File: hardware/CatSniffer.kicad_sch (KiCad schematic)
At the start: 76 parts, among them J1 Antenna, J2 Conn_01x06_Female, J3 Conn_01x06_Female, P1 USB_C_Plug_USB2.0, SW1 SW, U1 AP2112K-3.3, U2 RFSW8006QTR7, U3 ATSAMD21E18A, U4 0900PC15A0036, U5 0900FM15D0039, U6 SW409, U7 SX1262IMLTRT, U8 CC1352P1F3RGZT, Y1 48MHz, Y2 32.768kHz, Y3 32Mhz

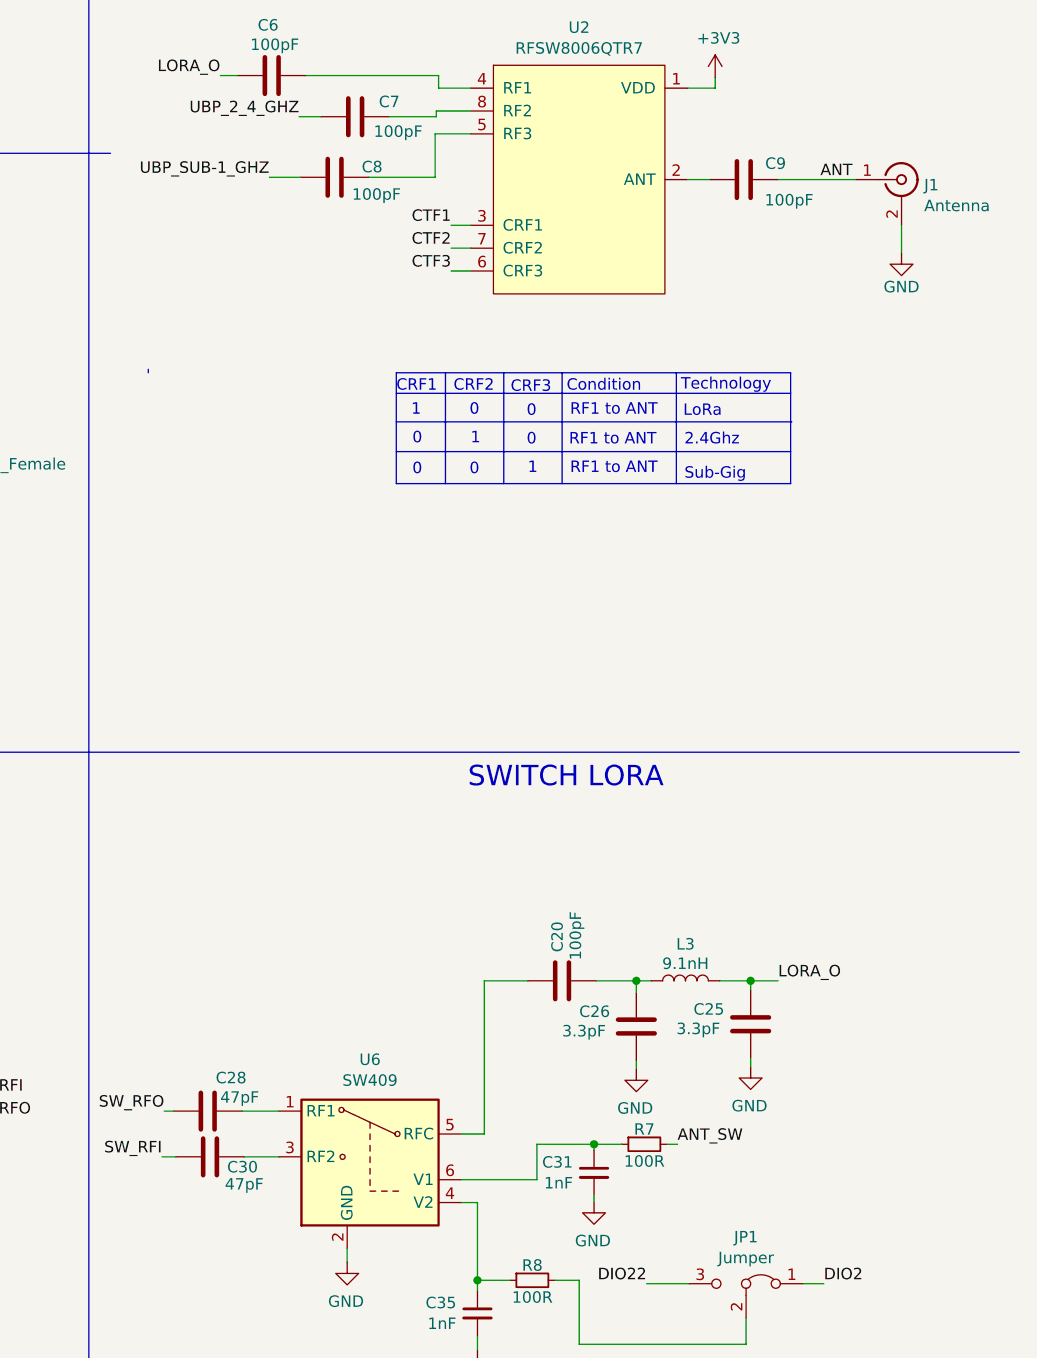
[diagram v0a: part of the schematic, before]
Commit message: update version
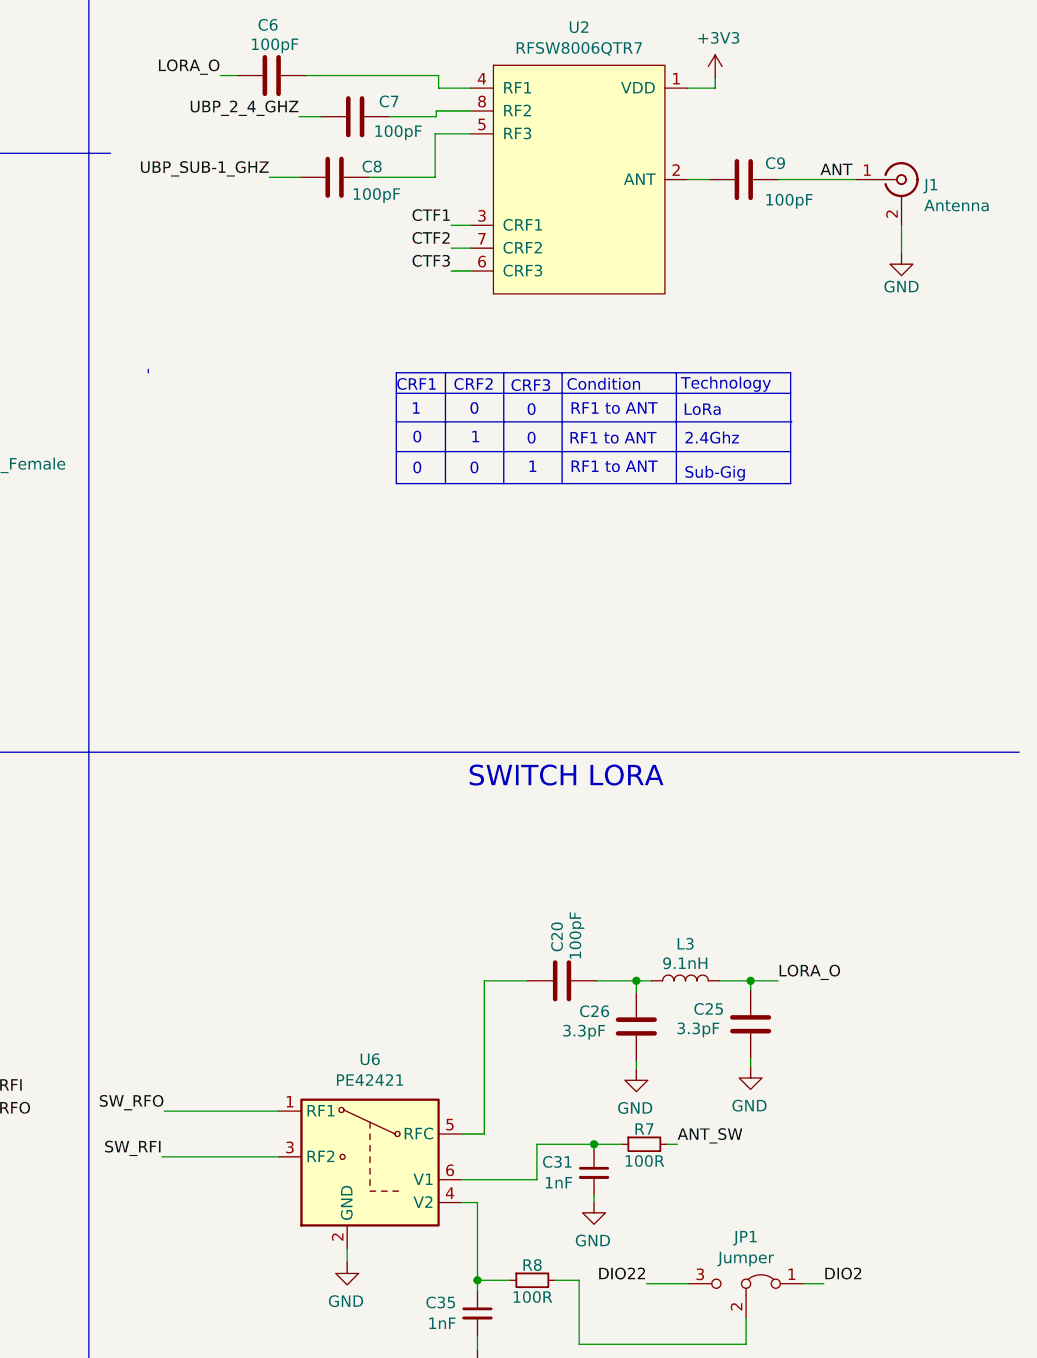
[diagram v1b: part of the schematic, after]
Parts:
- removed C28, C30: 47pF, Capacitor_SMD:C_0603_1608Metric, symbol CatSniffer-rescue:C-Device-CatStick-rescue-CatSniffer-rescue
- U6: value SW409 -> PE42421; footprint CatSniffer:SW409 -> Package_TO_SOT_SMD:SOT-363_SC-70-6; LCSC# C391968 -> -; manf# SW409 -> PE42421SCAA-Z; provedor LCSC -> Mouser
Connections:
- net SW_RFI: now also U6.3 (RF2)
- net SW_RFO: now also U6.1 (RF1)
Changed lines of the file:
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@@
     (title "CatSniffer")
     (date "2021-04-11")
-    (rev "1.0")
+    (rev "2.0")
     (company "ElectronicCats")
     (comment 3 "Edgar Herrera")
@@
     (stroke (width 0) (type default) (color 0 0 0 0))
   )
-  (wire (pts (xy 486.664 186.309) (xy 488.188 186.309))
-    (stroke (width 0) (type default) (color 0 0 0 0))
-  )
   (wire (pts (xy 303.403 50.673) (xy 316.103 50.673))
     (stroke (width 0) (type default) (color 0 0 0 0))
@@
     (stroke (width 0) (type default) (color 0 0 0 0))
   )
+  (wire (pts (xy 486.664 186.309) (xy 499.618 186.309))
+    (stroke (width 0) (type default) (color 0 0 0 0))
+  )
   (wire (pts (xy 314.198 192.024) (xy 312.039 192.024))
     (stroke (width 0) (type default) (color 0 0 0 0))
@@
     (stroke (width 0) (type default) (color 0 0 0 0))
   )
+  (wire (pts (xy 486.918 181.229) (xy 499.618 181.229))
+    (stroke (width 0) (type default) (color 0 0 0 0))
+  )
   (wire (pts (xy 548.64 166.751) (xy 552.069 166.751))
     (stroke (width 0) (type default) (color 0 0 0 0))
@@
     (stroke (width 0) (type default) (color 0 0 0 0))
   )
-  (wire (pts (xy 495.554 181.229) (xy 499.618 181.229))
-    (stroke (width 0) (type default) (color 0 0 0 0))
-  )
   (wire (pts (xy 357.124 169.164) (xy 357.124 164.719))
     (stroke (width 0) (type default) (color 0 0 0 0))
   )
-  (wire (pts (xy 495.808 186.309) (xy 499.618 186.309))
-    (stroke (width 0) (type default) (color 0 0 0 0))
-  )
   (polyline (pts (xy 531.114 99.187) (xy 531.114 111.506))
     (stroke (width 0) (type default) (color 0 0 0 0))
@@
     (stroke (width 0) (type default) (color 0 0 0 0))
   )
-  (wire (pts (xy 486.918 181.229) (xy 487.934 181.229))
-    (stroke (width 0) (type default) (color 0 0 0 0))
-  )
   (wire (pts (xy 177.038 166.37) (xy 172.339 166.37))
     (stroke (width 0) (type default) (color 0 0 0 0))
@@
     (pin "1")
   )
-  (symbol (lib_id "CatSniffer-rescue:C-Device-CatStick-rescue-CatSniffer-rescue") (at 491.744 181.229 90) (unit 1)
-    (in_bom yes) (on_board yes)
-    (property "Reference" "C28" (id 0) (at 496.062 177.546 90)
-      (effects (font (size 1.27 1.27)) (justify left))
-    )
-    (property "Value" "47pF" (id 1) (at 497.459 179.705 90)
-      (effects (font (size 1.27 1.27)) (justify left))
-    )
-    (property "Footprint" "Capacitor_SMD:C_0603_1608Metric" (id 2) (at 495.554 180.2638 0)
-      (effects (font (size 1.27 1.27)) hide)
-    )
-    (property "Datasheet" "" (id 3) (at 491.744 181.229 0))
-    (property "provedor" "LCSC" (id 4) (at 491.744 181.229 0)
-      (effects (font (size 1.27 1.27)) hide)
-    )
-    (property "LCSC#" "C519486" (id 5) (at 491.744 181.229 0)
-      (effects (font (size 1.27 1.27)) hide)
-    )
-    (property "manf#" "CC0603FRNPO9BN470" (id 6) (at 491.744 181.229 0)
-      (effects (font (size 1.27 1.27)) hide)
-    )
-    (pin "1")
-    (pin "2")
-  )
-  (symbol (lib_id "CatSniffer-rescue:C-Device-CatStick-rescue-CatSniffer-rescue") (at 491.998 186.309 90) (unit 1)
-    (in_bom yes) (on_board yes)
-    (property "Reference" "C30" (id 0) (at 497.332 187.452 90)
-      (effects (font (size 1.27 1.27)) (justify left))
-    )
-    (property "Value" "47pF" (id 1) (at 497.967 189.357 90)
-      (effects (font (size 1.27 1.27)) (justify left))
-    )
-    (property "Footprint" "Capacitor_SMD:C_0603_1608Metric" (id 2) (at 495.808 185.3438 0)
-      (effects (font (size 1.27 1.27)) hide)
-    )
-    (property "Datasheet" "" (id 3) (at 491.998 186.309 0))
-    (property "provedor" "LCSC" (id 4) (at 491.998 186.309 0)
-      (effects (font (size 1.27 1.27)) hide)
-    )
-    (property "LCSC#" "C519486" (id 5) (at 491.998 186.309 0)
-      (effects (font (size 1.27 1.27)) hide)
-    )
-    (property "manf#" "CC0603FRNPO9BN470" (id 6) (at 491.998 186.309 0)
-      (effects (font (size 1.27 1.27)) hide)
-    )
-    (pin "1")
-    (pin "2")
-  )
   (symbol (lib_id "CatSniffer-rescue:C-Device-CatStick-rescue-CatSniffer-rescue") (at 539.369 171.831 0) (unit 1)
     (in_bom yes) (on_board yes)
@@
     (in_bom yes) (on_board yes)
     (property "Reference" "U6" (id 0) (at 509.778 175.514 0))
-    (property "Value" "SW409" (id 1) (at 509.778 177.8254 0))
-    (property "Footprint" "CatSniffer:SW409" (id 2) (at 509.778 183.769 0)
+    (property "Value" "PE42421" (id 1) (at 509.778 177.8254 0))
+    (property "Footprint" "Package_TO_SOT_SMD:SOT-363_SC-70-6" (id 2) (at 509.778 183.769 0)
       (effects (font (size 1.27 1.27)) hide)
     )
-    (property "Datasheet" "https://datasheet.lcsc.com/lcsc/1912111437_RFIC-SW409_C391968.pdf" (id 3) (at 509.778 183.769 0)
+    (property "Datasheet" "https://www.mouser.mx/datasheet/2/281/pe42421ds-1671115.pdf" (id 3) (at 509.778 183.769 0)
       (effects (font (size 1.27 1.27)) hide)
     )
-    (property "LCSC#" "C391968" (id 4) (at 509.778 186.309 0)
+    (property "LCSC#" "-" (id 4) (at 509.778 186.309 0)
       (effects (font (size 1.27 1.27)) hide)
     )
-    (property "manf#" "SW409" (id 5) (at 509.778 186.309 0)
+    (property "manf#" "PE42421SCAA-Z" (id 5) (at 509.778 186.309 0)
       (effects (font (size 1.27 1.27)) hide)
     )
-    (property "provedor" "LCSC" (id 6) (at 509.778 186.309 0)
+    (property "provedor" "Mouser" (id 6) (at 509.778 186.309 0)
       (effects (font (size 1.27 1.27)) hide)
     )
@@
       (reference "C27") (unit 1) (value "100pF") (footprint "Capacitor_SMD:C_0603_1608Metric")
     )
-    (path "/00000000-0000-0000-0000-000060977a2f"
-      (reference "C28") (unit 1) (value "47pF") (footprint "Capacitor_SMD:C_0603_1608Metric")
-    )
     (path "/00000000-0000-0000-0000-000060ea4035"
       (reference "C29") (unit 1) (value "0.1uF") (footprint "Capacitor_SMD:C_0603_1608Metric")
     )
-    (path "/00000000-0000-0000-0000-000060977e80"
-      (reference "C30") (unit 1) (value "47pF") (footprint "Capacitor_SMD:C_0603_1608Metric")
-    )
     (path "/00000000-0000-0000-0000-000060cf4963"
       (reference "C31") (unit 1) (value "1nF") (footprint "Capacitor_SMD:C_0603_1608Metric")
@@
     )
     (path "/00000000-0000-0000-0000-000060fa8e32"
-      (reference "U6") (unit 1) (value "SW409") (footprint "CatSniffer:SW409")
+      (reference "U6") (unit 1) (value "PE42421") (footprint "Package_TO_SOT_SMD:SOT-363_SC-70-6")
     )
     (path "/00000000-0000-0000-0000-000060bf3807"

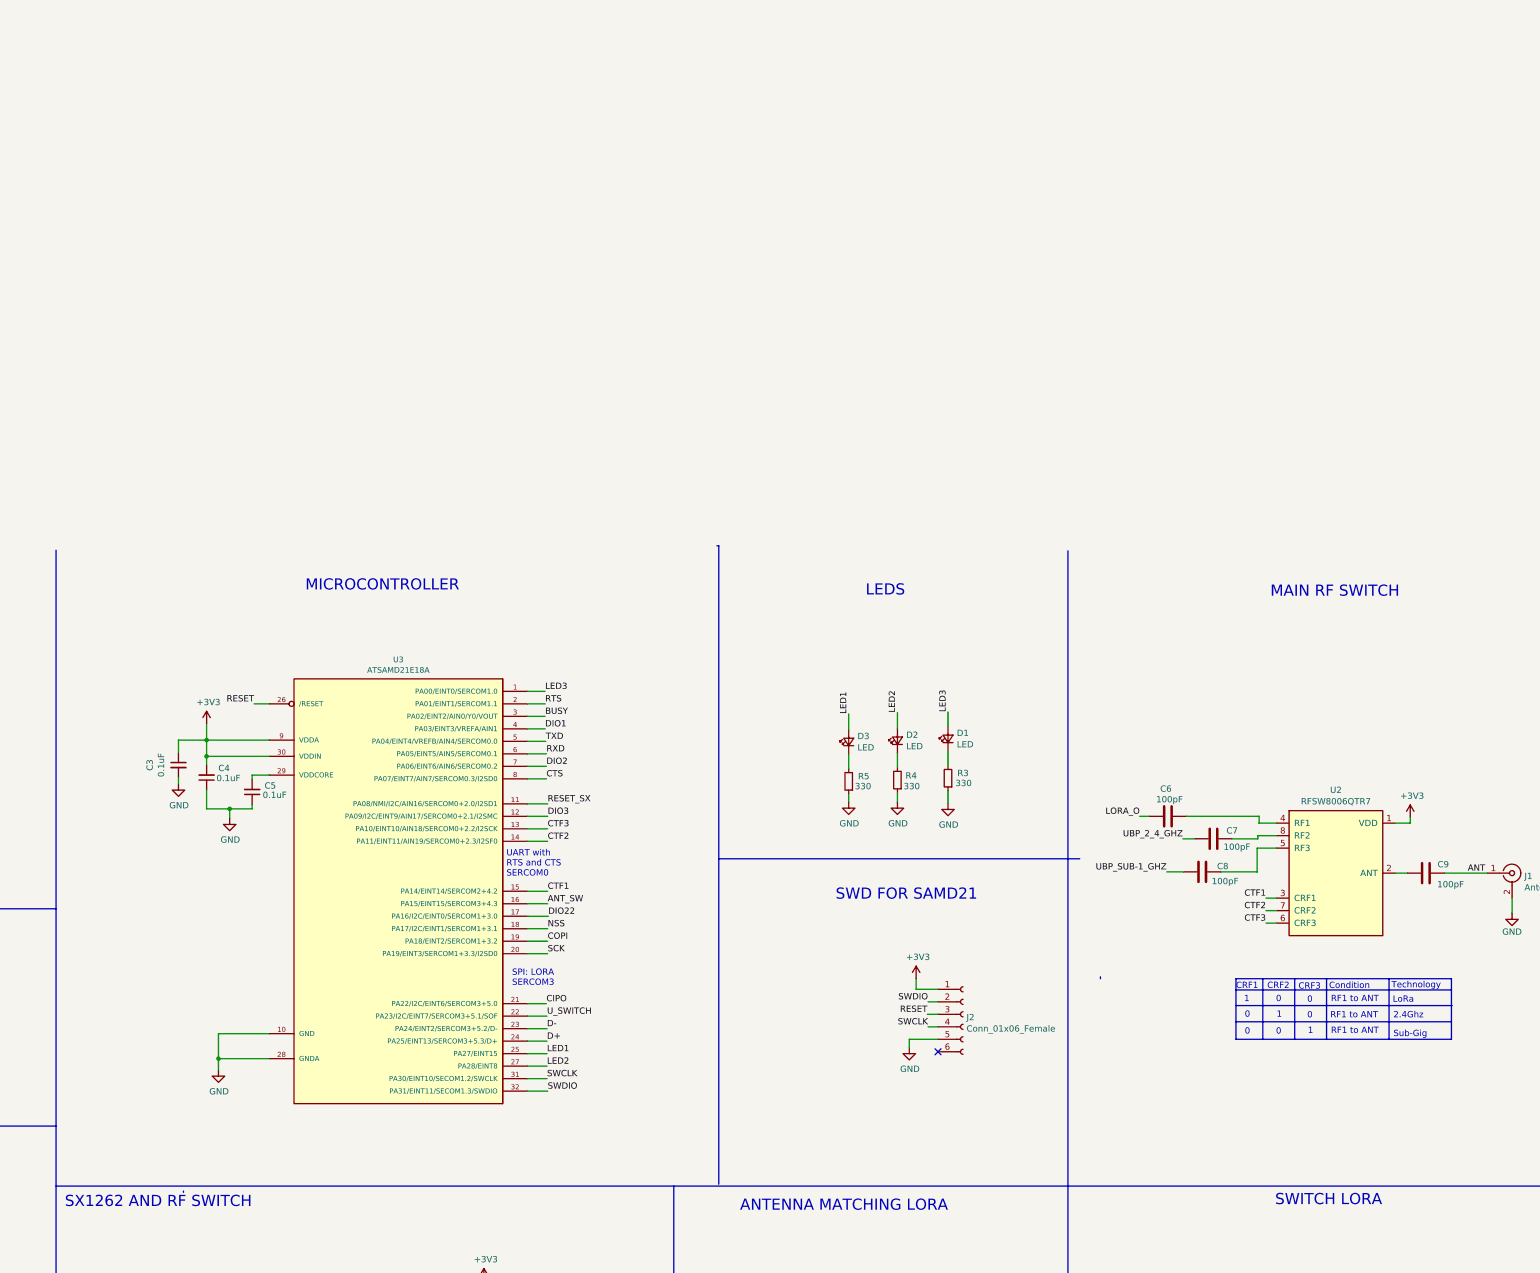
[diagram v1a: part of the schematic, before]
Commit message: Init RP2040
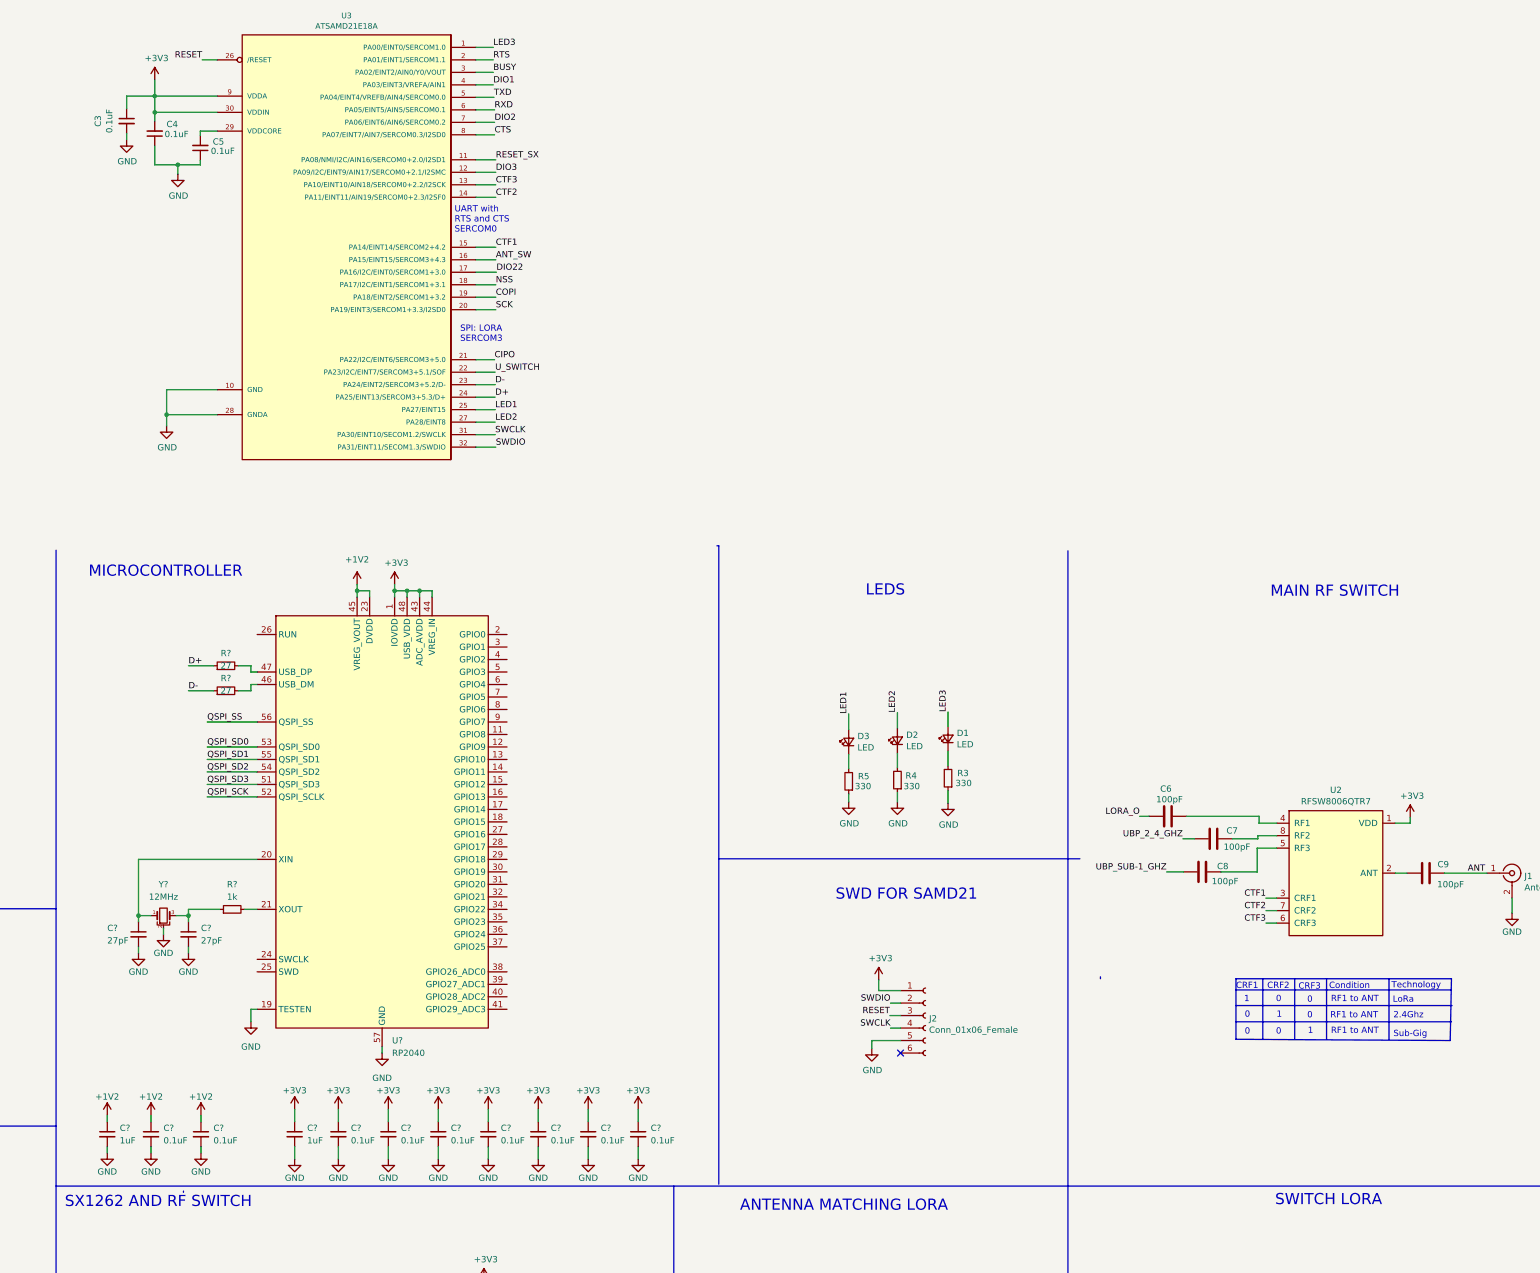
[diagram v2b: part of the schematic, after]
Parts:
- added C? (x2): 1uF, symbol Device:C_Small
- added C? (x2): 27pF, symbol Device:C_Small
- added C? (x9): 0.1uF, symbol Device:C_Small
- added R? (x2): 27, symbol Device:R_Small
- added R?: 1k, symbol Device:R_Small
- added U?: RP2040, Package_DFN_QFN:QFN-56-1EP_7x7mm_P0.4mm_EP3.2x3.2mm, symbol MCU_RaspberryPi:RP2040
- added Y?: 12MHz, symbol Device:Crystal_GND2_Small
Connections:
- net +3V3: now also C?.1, C?.1, C?.1, C?.1, C?.1, C?.1, C?.1, C?.1, U?.1 (IOVDD), U?.10 (IOVDD), U?.22 (IOVDD), U?.33 (IOVDD), U?.42 (IOVDD), U?.43 (ADC_AVDD), U?.44 (VREG_IN), U?.48 (USB_VDD), U?.49 (IOVDD)
- net D+: now also R?.1
- net D-: now also R?.1
- net GND: now also C?.2, C?.2, C?.2, C?.2, C?.2, C?.2, C?.2, C?.2, C?.2, C?.2, C?.2, C?.2, C?.2, U?.19 (TESTEN), U?.57 (GND), Y?.2
- new net: C?.1, R?.1, Y?.3
- new net: R?.2, U?.47 (USB_DP)
- new net: C?.1, U?.20 (XIN), Y?.1
- new net: R?.2, U?.21 (XOUT)
- new net: R?.2, U?.46 (USB_DM)
- new net +1V2: C?.1, C?.1, C?.1, U?.23 (DVDD), U?.45 (VREG_VOUT), U?.50 (DVDD)
- new net QSPI_SCK: U?.52 (QSPI_SCLK)
- new net QSPI_SD0: U?.53 (QSPI_SD0)
- new net QSPI_SD1: U?.55 (QSPI_SD1)
- new net QSPI_SD2: U?.54 (QSPI_SD2)
- new net QSPI_SD3: U?.51 (QSPI_SD3)
- new net QSPI_SS: U?.56 (QSPI_SS)
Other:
- moved on the sheet: C3, C4, C5, J2, U3
